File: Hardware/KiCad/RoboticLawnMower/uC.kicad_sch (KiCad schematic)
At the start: 1 part, among them U2 AVR128DB48x-xPT

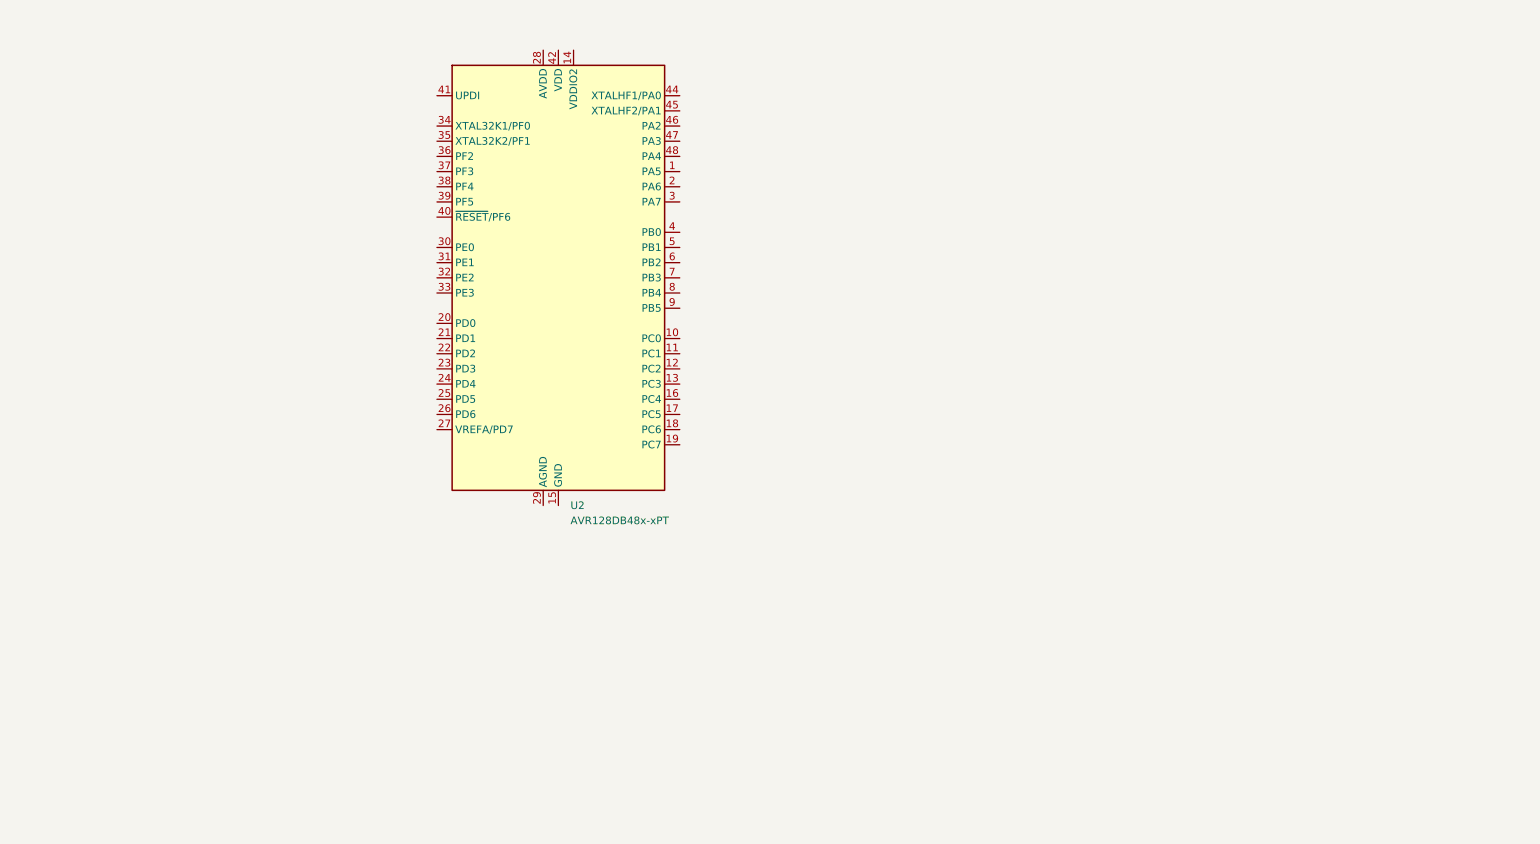
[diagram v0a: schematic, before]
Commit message: layout update
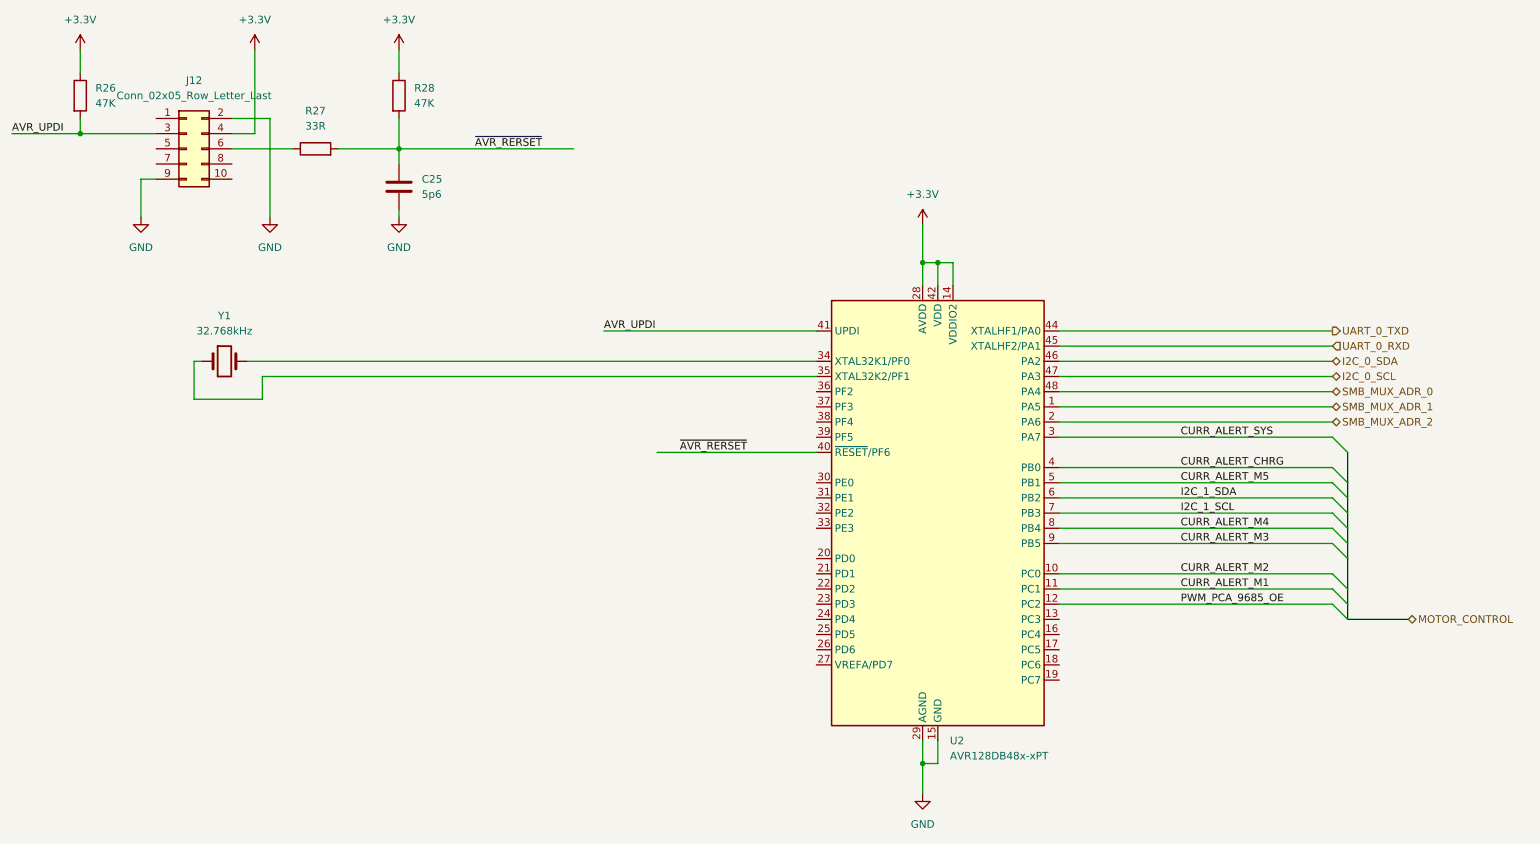
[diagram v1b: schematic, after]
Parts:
- added C25: 5p6, Capacitor_SMD:C_0603_1608Metric, symbol Device:C
- added J12: Conn_02x05_Row_Letter_Last, symbol Connector_Generic:Conn_02x05_Odd_Even
- added R26, R28: 47K, Resistor_SMD:R_0603_1608Metric, symbol Device:R
- added R27: 33R, Resistor_SMD:R_0603_1608Metric, symbol Device:R
- added Y1: 32.768kHz, symbol Device:Crystal
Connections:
- net SMB_MUX_ADR_1: now reaches U2.1 (PA5)
- net CURR_ALERT_M2: now reaches U2.10 (PC0)
- net CURR_ALERT_M1: now reaches U2.11 (PC1)
- net PWM_PCA_9685_OE: now reaches U2.12 (PC2)
- net +3.3V: now reaches U2.14 (VDDIO2)
- net +3.3V: now also U2.28 (AVDD), U2.42 (VDD), J12.4 (Pin_4), R26.1, R28.1
- net GND: now reaches U2.15 (GND), U2.43 (GND)
- net GND: now also U2.29 (AGND), C25.2, J12.2 (Pin_2), J12.9 (Pin_9)
- net SMB_MUX_ADR_2: now reaches U2.2 (PA6)
- net CURR_ALERT_SYS: now reaches U2.3 (PA7)
- net at U2.34 (XTAL32K1/PF0): now also Y1.2
- net at U2.35 (XTAL32K2/PF1): now also Y1.1
- net CURR_ALERT_CHRG: now reaches U2.4 (PB0)
- net ~{AVR_RERSET}: now reaches U2.40 (~{RESET}/PF6)
- net ~{AVR_RERSET}: now also C25.1, R27.2, R28.2
- net AVR_UPDI: now reaches U2.41 (UPDI)
- net AVR_UPDI: now also J12.3 (Pin_3), R26.2
- net UART_0_TXD: now reaches U2.44 (XTALHF1/PA0)
- net UART_0_RXD: now reaches U2.45 (XTALHF2/PA1)
- net I2C_0_SDA: now reaches U2.46 (PA2)
- net I2C_0_SCL: now reaches U2.47 (PA3)
- net SMB_MUX_ADR_0: now reaches U2.48 (PA4)
- net CURR_ALERT_M5: now reaches U2.5 (PB1)
- net I2C_1_SDA: now reaches U2.6 (PB2)
- net I2C_1_SCL: now reaches U2.7 (PB3)
- net CURR_ALERT_M4: now reaches U2.8 (PB4)
- net CURR_ALERT_M3: now reaches U2.9 (PB5)
- new net: J12.6 (Pin_6), R27.1
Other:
- moved on the sheet: U2
